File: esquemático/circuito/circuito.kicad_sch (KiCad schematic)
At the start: 6 parts, among them K1 Módulo Relé, M1 Servo Motor 180, M2 Servo Motor 360, Q1 BC107, U1 Olimex_MOD-WIFI-ESP8266-DEV

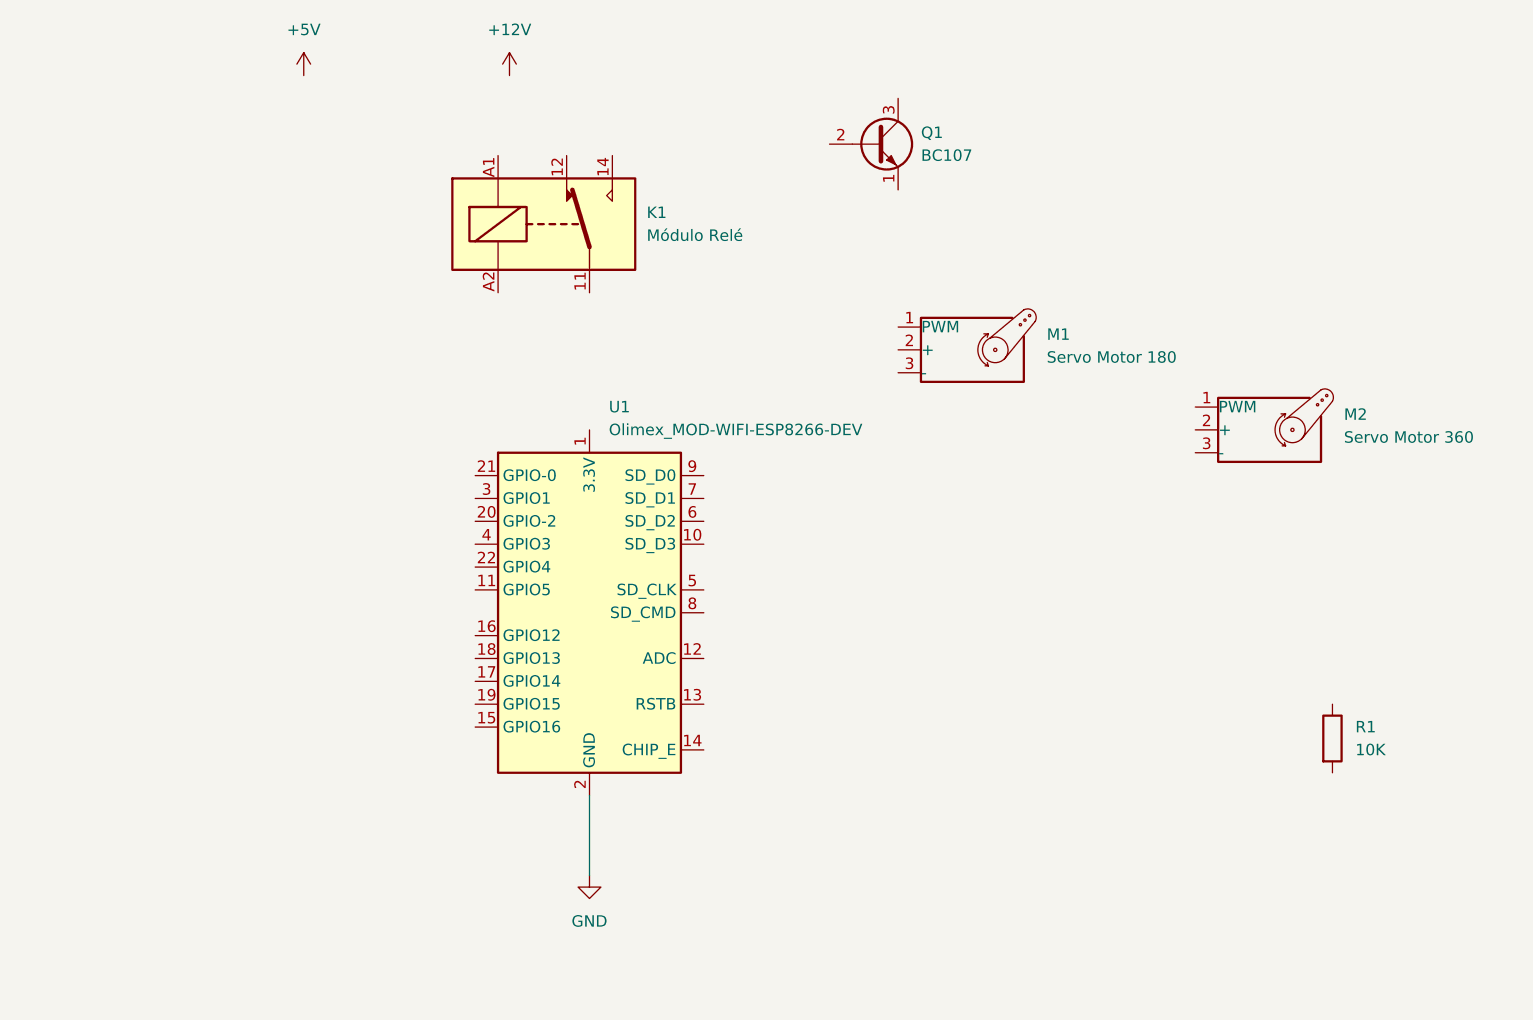
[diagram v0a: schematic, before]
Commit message: Correções e finalização do circuito
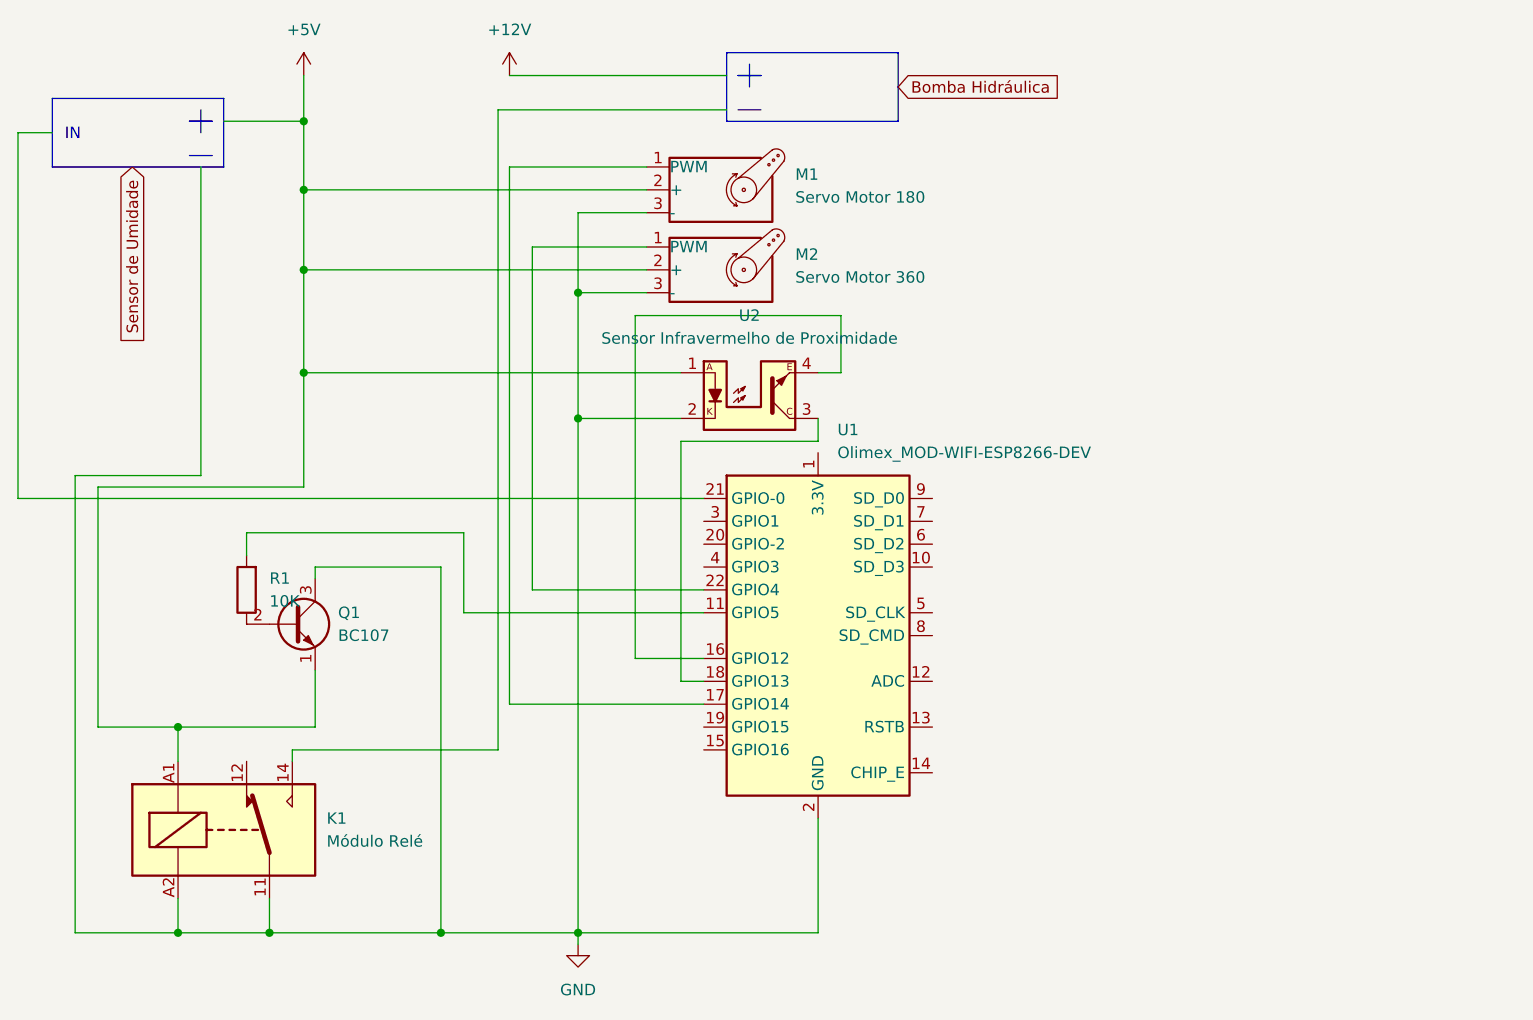
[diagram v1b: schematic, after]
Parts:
- added U2: Sensor Infravermelho de Proximidade, OptoDevice:Everlight_ITR9608-F, symbol Sensor_Proximity:ITR9608-F
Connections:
- net +5V: now also K1.A1, M1.2 (+), M2.2 (+), Q1.1 (E), U2.1
- net GND: now also K1.11, K1.A2, M1.3 (-), M2.3 (-), Q1.3 (C), U2.2
- net at U1.11 (GPIO5): now also R1.2
- net at U1.16 (GPIO12): now also U2.4
- net at U1.17 (GPIO14): now also M1.1 (PWM)
- net at U1.18 (GPIO13): now also U2.3
- net at U1.22 (GPIO4): now also M2.1 (PWM)
- net at R1.1: now also Q1.2 (B)
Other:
- note added: "IN"
- moved on the sheet: K1, M1, M2, Q1, R1, U1
